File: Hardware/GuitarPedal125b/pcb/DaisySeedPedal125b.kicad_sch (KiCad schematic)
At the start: 13 parts, among them J1 POWER_JACK, J11 Conn_01x05_Pin, J12 Conn_01x02_Pin, J13 Conn_01x01_Pin, J2 AUDIO_IN_LEFT, J3 AUDIO_IN_RIGHT, J4 AUDIO_OUT_LEFT, J5 AUDIO_OUT_RIGHT, J6 MIDI_IN, J7 MIDI_OUT, J8 Conn_01x20_Socket, J9 Conn_01x20_Socket

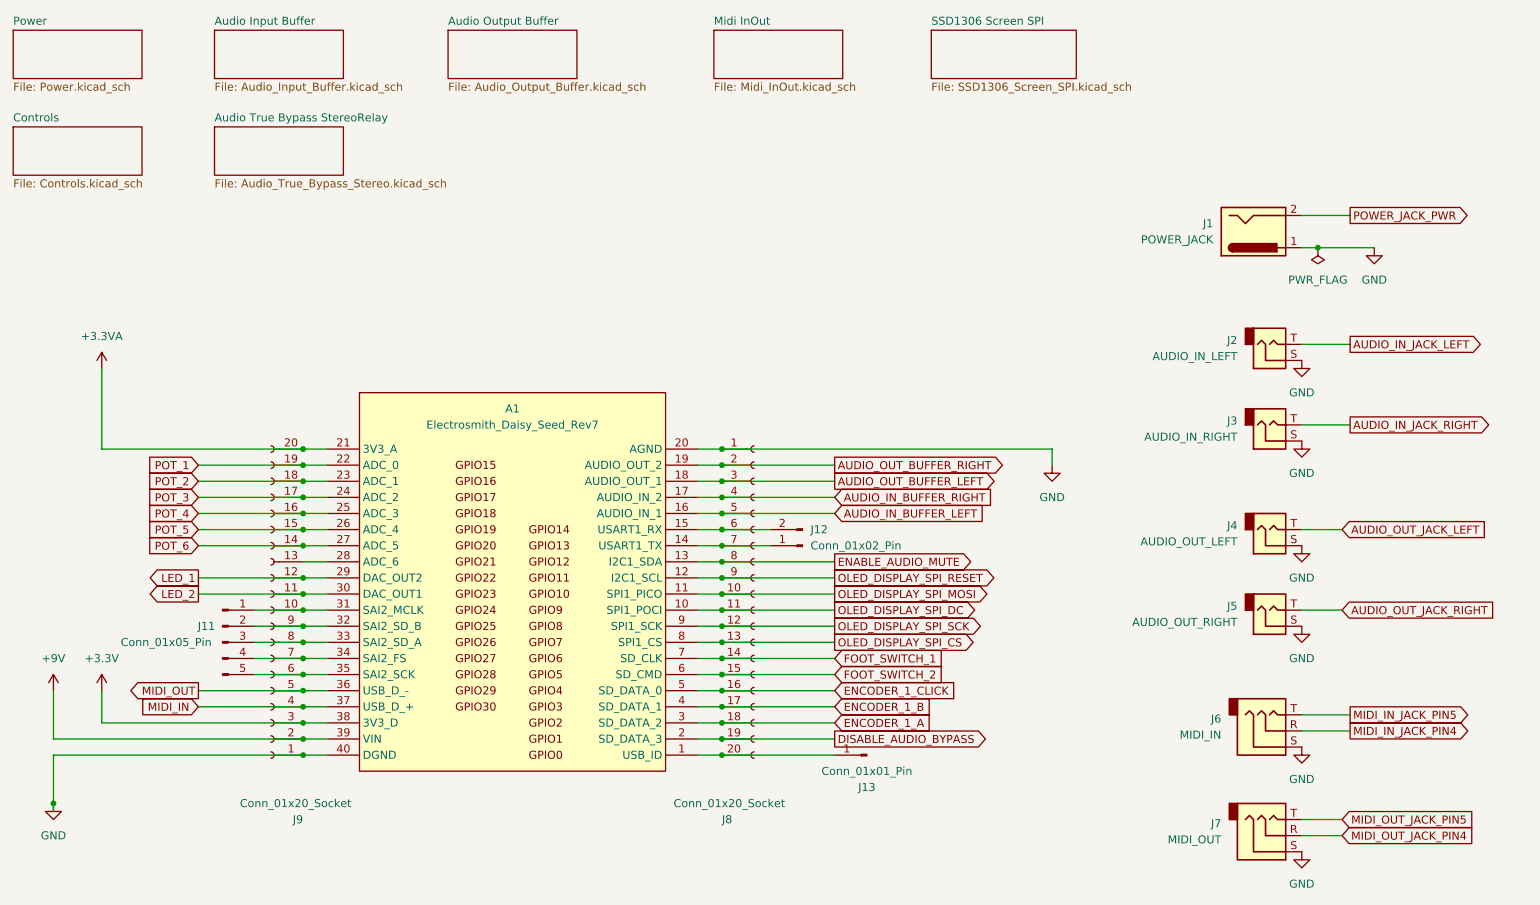
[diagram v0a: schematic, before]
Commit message: More work on layout
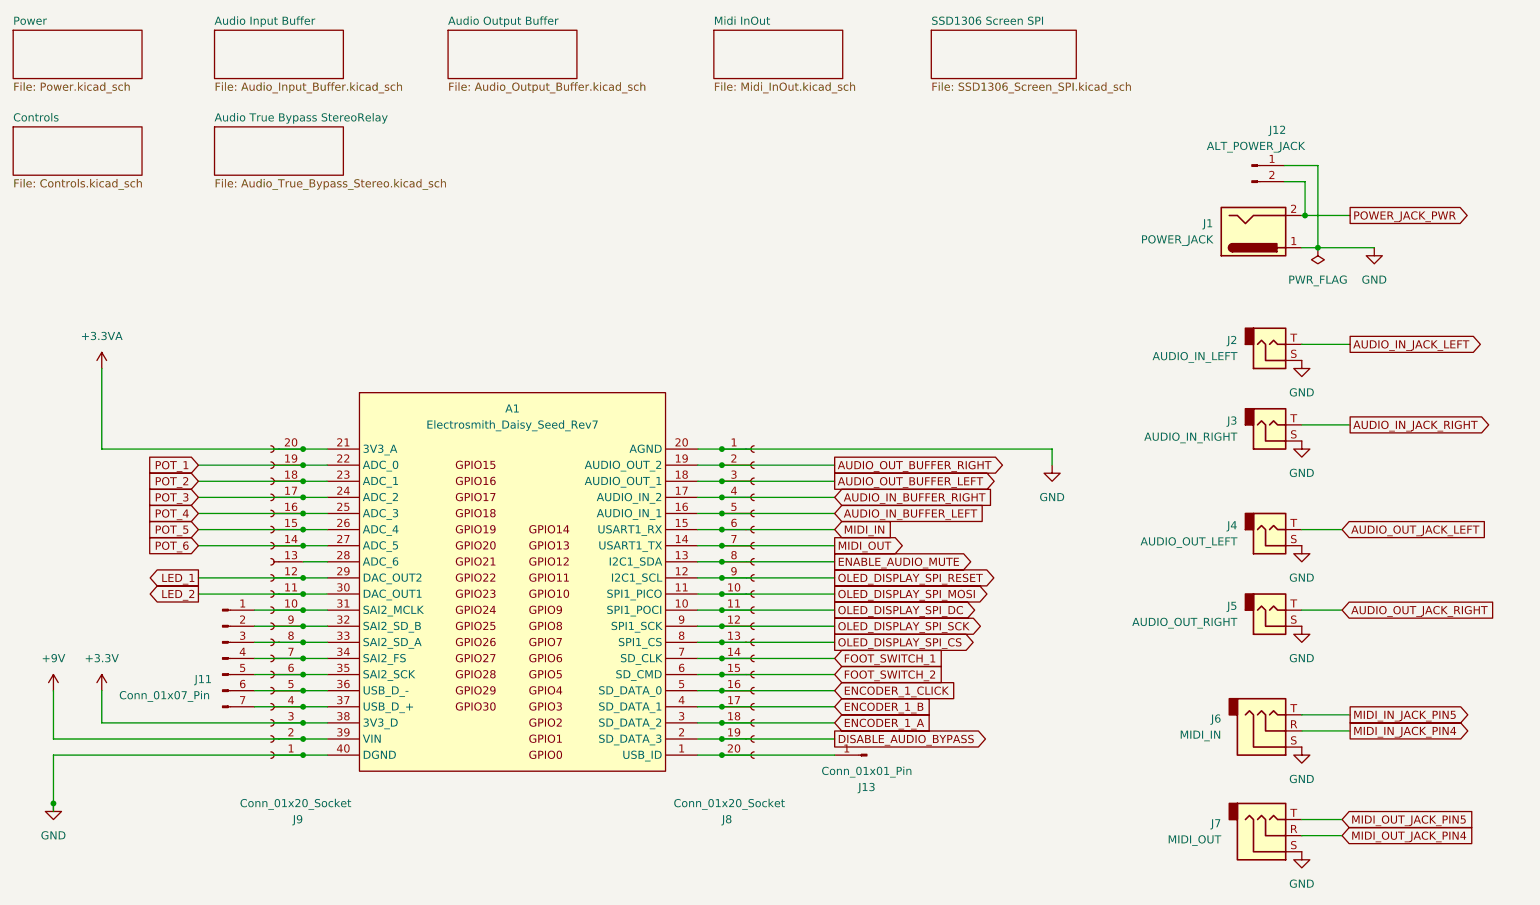
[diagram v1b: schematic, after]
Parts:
- removed J11: Conn_01x05_Pin, Connector_PinHeader_2.54mm:PinHeader_1x05_P2.54mm_Vertical, symbol Connector:Conn_01x05_Pin
- added J11: Conn_01x07_Pin, Connector_PinHeader_2.54mm:PinHeader_1x07_P2.54mm_Vertical, symbol Connector:Conn_01x07_Pin
- J12: value Conn_01x02_Pin -> ALT_POWER_JACK; footprint Connector_PinHeader_2.54mm:PinHeader_1x02_P2.54mm_Vertical -> GuitarPedal125B:Generic_Pads_Power
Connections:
- net GND: now also J12.1 (Pin_1)
- net MIDI_IN: now also A1.15 (USART1_RX), J8.6 (Pin_6); no longer A1.37 (USB_D_+), J9.4 (Pin_4)
- net MIDI_OUT: now also A1.14 (USART1_TX), J8.7 (Pin_7); no longer A1.36 (USB_D_-), J9.5 (Pin_5)
- net POWER_JACK_PWR: now also J12.2 (Pin_2)
- net at A1.31 (SAI2_MCLK), J9.10 (Pin_10): now also J11.1 (Pin_1)
- net at A1.32 (SAI2_SD_B), J9.9 (Pin_9): now also J11.2 (Pin_2)
- net at A1.33 (SAI2_SD_A), J9.8 (Pin_8): now also J11.3 (Pin_3)
- net at A1.34 (SAI2_FS), J9.7 (Pin_7): now also J11.4 (Pin_4)
- net at A1.35 (SAI2_SCK), J9.6 (Pin_6): now also J11.5 (Pin_5)
- new net: A1.36 (USB_D_-), J11.6 (Pin_6), J9.5 (Pin_5)
- new net: A1.37 (USB_D_+), J11.7 (Pin_7), J9.4 (Pin_4)
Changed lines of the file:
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@@
   (junction (at 130.81 120.65) (diameter 0) (color 0 0 0 0)
   )
+  (junction (at 64.77 123.19) (diameter 0) (color 0 0 0 0)
+  )
   (junction (at 64.77 105.41) (diameter 0) (color 0 0 0 0)
   )
@@
   (junction (at 130.81 105.41) (diameter 0) (color 0 0 0 0)
   )
+  (junction (at 130.81 128.27) (diameter 0) (color 0 0 0 0)
+  )
+  (junction (at 130.81 90.17) (diameter 0) (color 0 0 0 0)
+  )
+  (junction (at 130.81 100.33) (diameter 0) (color 0 0 0 0)
+  )
   (junction (at 64.77 125.73) (diameter 0) (color 0 0 0 0)
   )
-  (junction (at 130.81 128.27) (diameter 0) (color 0 0 0 0)
-  )
-  (junction (at 130.81 90.17) (diameter 0) (color 0 0 0 0)
-  )
-  (junction (at 130.81 100.33) (diameter 0) (color 0 0 0 0)
-  )
   (junction (at 64.77 130.81) (diameter 0) (color 0 0 0 0)
   )
@@
   (junction (at 64.77 100.33) (diameter 0) (color 0 0 0 0)
   )
+  (junction (at 222.758 48.26) (diameter 0) (color 0 0 0 0)
+  )
   (junction (at 130.81 115.57) (diameter 0) (color 0 0 0 0)
   )
-  (junction (at 64.77 123.19) (diameter 0) (color 0 0 0 0)
-  )
   (junction (at 130.81 133.35) (diameter 0) (color 0 0 0 0)
   )
@@
     (stroke (width 0) (type default))
   )
-  (wire (pts (xy 130.81 97.79) (xy 138.43 97.79))
-    (stroke (width 0) (type default))
-  )
   (wire (pts (xy 222.25 110.49) (xy 228.6 110.49))
     (stroke (width 0) (type default))
@@
     (stroke (width 0) (type default))
   )
-  (wire (pts (xy 222.25 48.26) (xy 229.87 48.26))
+  (wire (pts (xy 222.25 48.26) (xy 222.758 48.26))
     (stroke (width 0) (type default))
   )
@@
     (stroke (width 0) (type default))
   )
+  (wire (pts (xy 222.758 42.926) (xy 222.758 48.26))
+    (stroke (width 0) (type default))
+  )
   (wire (pts (xy 64.77 110.49) (xy 68.58 110.49))
     (stroke (width 0) (type default))
@@
     (stroke (width 0) (type default))
   )
-  (wire (pts (xy 48.26 123.19) (xy 64.77 123.19))
-    (stroke (width 0) (type default))
-  )
   (wire (pts (xy 127 128.27) (xy 130.81 128.27))
     (stroke (width 0) (type default))
@@
     (stroke (width 0) (type default))
   )
+  (wire (pts (xy 57.15 125.73) (xy 64.77 125.73))
+    (stroke (width 0) (type default))
+  )
   (wire (pts (xy 64.77 130.81) (xy 68.58 130.81))
     (stroke (width 0) (type default))
@@
     (stroke (width 0) (type default))
   )
-  (wire (pts (xy 48.26 125.73) (xy 64.77 125.73))
-    (stroke (width 0) (type default))
-  )
   (wire (pts (xy 127 87.63) (xy 130.81 87.63))
     (stroke (width 0) (type default))
@@
     (stroke (width 0) (type default))
   )
+  (wire (pts (xy 224.79 40.386) (xy 224.79 53.34))
+    (stroke (width 0) (type default))
+  )
   (wire (pts (xy 127 133.35) (xy 130.81 133.35))
     (stroke (width 0) (type default))
@@
     (stroke (width 0) (type default))
   )
+  (wire (pts (xy 57.15 123.19) (xy 64.77 123.19))
+    (stroke (width 0) (type default))
+  )
+  (wire (pts (xy 219.456 42.926) (xy 222.758 42.926))
+    (stroke (width 0) (type default))
+  )
   (wire (pts (xy 222.25 127) (xy 229.87 127))
     (stroke (width 0) (type default))
@@
     (stroke (width 0) (type default))
   )
+  (wire (pts (xy 130.81 100.33) (xy 148.59 100.33))
+    (stroke (width 0) (type default))
+  )
+  (wire (pts (xy 130.81 97.79) (xy 148.59 97.79))
+    (stroke (width 0) (type default))
+  )
   (wire (pts (xy 48.26 107.95) (xy 64.77 107.95))
     (stroke (width 0) (type default))
@@
     (stroke (width 0) (type default))
   )
+  (wire (pts (xy 222.758 48.26) (xy 229.87 48.26))
+    (stroke (width 0) (type default))
+  )
   (wire (pts (xy 130.81 110.49) (xy 148.59 110.49))
     (stroke (width 0) (type default))
@@
     (stroke (width 0) (type default))
   )
-  (wire (pts (xy 130.81 100.33) (xy 138.43 100.33))
-    (stroke (width 0) (type default))
-  )
   (wire (pts (xy 25.4 123.19) (xy 25.4 130.81))
     (stroke (width 0) (type default))
@@
     (stroke (width 0) (type default))
   )
+  (wire (pts (xy 219.456 40.386) (xy 224.79 40.386))
+    (stroke (width 0) (type default))
+  )
   (wire (pts (xy 64.77 113.03) (xy 68.58 113.03))
     (stroke (width 0) (type default))
@@
     )
   )
-  (global_label "MIDI_IN" (shape input) (at 48.26 125.73 180) (fields_autoplaced)
-    (effects (font (size 1.27 1.27)) (justify right))
-    (property "Intersheetrefs" "${INTERSHEET_REFS}" (at 38.4409 125.73 0)
-      (effects (font (size 1.27 1.27)) (justify right) hide)
+  (global_label "MIDI_IN" (shape input) (at 148.59 97.79 0) (fields_autoplaced)
+    (effects (font (size 1.27 1.27)) (justify left))
+    (property "Intersheetrefs" "${INTERSHEET_REFS}" (at 158.4091 97.79 0)
+      (effects (font (size 1.27 1.27)) (justify left) hide)
     )
   )
@@
     )
   )
-  (global_label "MIDI_OUT" (shape output) (at 48.26 123.19 180) (fields_autoplaced)
-    (effects (font (size 1.27 1.27)) (justify right))
-    (property "Intersheetrefs" "${INTERSHEET_REFS}" (at 36.7476 123.19 0)
-      (effects (font (size 1.27 1.27)) (justify right) hide)
+  (global_label "MIDI_OUT" (shape output) (at 148.59 100.33 0) (fields_autoplaced)
+    (effects (font (size 1.27 1.27)) (justify left))
+    (property "Intersheetrefs" "${INTERSHEET_REFS}" (at 160.1024 100.33 0)
+      (effects (font (size 1.27 1.27)) (justify left) hide)
     )
   )
@@
     )
   )
+  (symbol (lib_id "Connector:Conn_01x07_Pin") (at 52.07 118.11 0) (unit 1)
+    (in_bom yes) (on_board yes) (dnp no)
+    (property "Reference" "J11" (at 49.022 121.412 0)
+      (effects (font (size 1.27 1.27)))
+    )
+    (property "Value" "Conn_01x07_Pin" (at 42.926 123.952 0)
+      (effects (font (size 1.27 1.27)))
+    )
+    (property "Footprint" "Connector_PinHeader_2.54mm:PinHeader_1x07_P2.54mm_Vertical" (at 52.07 118.11 0)
+      (effects (font (size 1.27 1.27)) hide)
+    )
+    (property "Datasheet" "~" (at 52.07 118.11 0)
+      (effects (font (size 1.27 1.27)) hide)
+    )
+    (pin "1")
+    (pin "6")
+    (pin "3")
+    (pin "4")
+    (pin "2")
+    (pin "5")
+    (pin "7")
+    (instances
+      (project "DaisySeedPedal125b"
+        (path "/1d54e6f4-7c7a-4f03-b2db-a136bdff5b99"
+          (reference "J11") (unit 1)
+        )
+      )
+    )
+  )
   (symbol (lib_id "Connector_Audio:AudioJack2") (at 217.17 81.28 0) (mirror x) (unit 1)
     (in_bom yes) (on_board yes) (dnp no)
@@
         (path "/1d54e6f4-7c7a-4f03-b2db-a136bdff5b99"
           (reference "#PWR0111") (unit 1)
-        )
-      )
-    )
-  )
-  (symbol (lib_id "Connector:Conn_01x02_Pin") (at 143.51 100.33 180) (unit 1)
-    (in_bom yes) (on_board yes) (dnp no) (fields_autoplaced)
-    (property "Reference" "J12" (at 144.78 97.79 0)
-      (effects (font (size 1.27 1.27)) (justify right))
-    )
-    (property "Value" "Conn_01x02_Pin" (at 144.78 100.33 0)
-      (effects (font (size 1.27 1.27)) (justify right))
-    )
-    (property "Footprint" "Connector_PinHeader_2.54mm:PinHeader_1x02_P2.54mm_Vertical" (at 143.51 100.33 0)
-      (effects (font (size 1.27 1.27)) hide)
-    )
-    (property "Datasheet" "~" (at 143.51 100.33 0)
-      (effects (font (size 1.27 1.27)) hide)
-    )
-    (pin "1")
-    (pin "2")
-    (instances
-      (project "DaisySeedPedal125b"
-        (path "/1d54e6f4-7c7a-4f03-b2db-a136bdff5b99"
-          (reference "J12") (unit 1)
         )
       )
@@
     )
   )
+  (symbol (lib_id "Connector:Conn_01x02_Pin") (at 214.376 40.386 0) (unit 1)
+    (in_bom yes) (on_board yes) (dnp no)
+    (property "Reference" "J12" (at 218.44 34.798 0)
+      (effects (font (size 1.27 1.27)))
+    )
+    (property "Value" "ALT_POWER_JACK" (at 215.011 37.338 0)
+      (effects (font (size 1.27 1.27)))
+    )
+    (property "Footprint" "GuitarPedal125B:Generic_Pads_Power" (at 214.376 40.386 0)
+      (effects (font (size 1.27 1.27)) hide)
+    )
+    (property "Datasheet" "~" (at 214.376 40.386 0)
+      (effects (font (size 1.27 1.27)) hide)
+    )
+    (pin "1")
+    (pin "2")
+    (instances
+      (project "DaisySeedPedal125b"
+        (path "/1d54e6f4-7c7a-4f03-b2db-a136bdff5b99"
+          (reference "J12") (unit 1)
+        )
+      )
+    )
+  )
   (symbol (lib_id "power:GND") (at 222.25 100.33 0) (unit 1)
     (in_bom yes) (on_board yes) (dnp no) (fields_autoplaced)
@@
         )
       )
-    )
-  )
-  (symbol (lib_id "Connector:Conn_01x05_Pin") (at 52.07 115.57 0) (unit 1)
-    (in_bom yes) (on_board yes) (dnp no)
-    (property "Reference" "J11" (at 49.53 113.03 0)
-      (effects (font (size 1.27 1.27)))
-    )
-    (property "Value" "Conn_01x05_Pin" (at 43.18 115.57 0)
-      (effects (font (size 1.27 1.27)))
-    )
-    (property "Footprint" "Connector_PinHeader_2.54mm:PinHeader_1x05_P2.54mm_Vertical" (at 52.07 115.57 0)
-      (effects (font (size 1.27 1.27)) hide)
-    )
-    (property "Datasheet" "~" (at 52.07 115.57 0)
-      (effects (font (size 1.27 1.27)) hide)
-    )
-    (pin "1")
-    (pin "2")
-    (pin "4")
-    (pin "3")
-    (pin "5")
-    (instances
-      (project "DaisySeedPedal125b"
-        (path "/1d54e6f4-7c7a-4f03-b2db-a136bdff5b99"
-          (reference "J11") (unit 1)
-        )
-      )
